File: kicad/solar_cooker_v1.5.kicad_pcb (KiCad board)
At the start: 2 copper layers, 160.5 x 77.2 mm, 20 parts, among them J1 Pt100, J2 microSD, J3 clock_module, J4 Pt100, J5 BME680, J6 GPS, J7 Pt100, J8 display, U1 anemometer, U2 AM2315C, U3 pyranometer

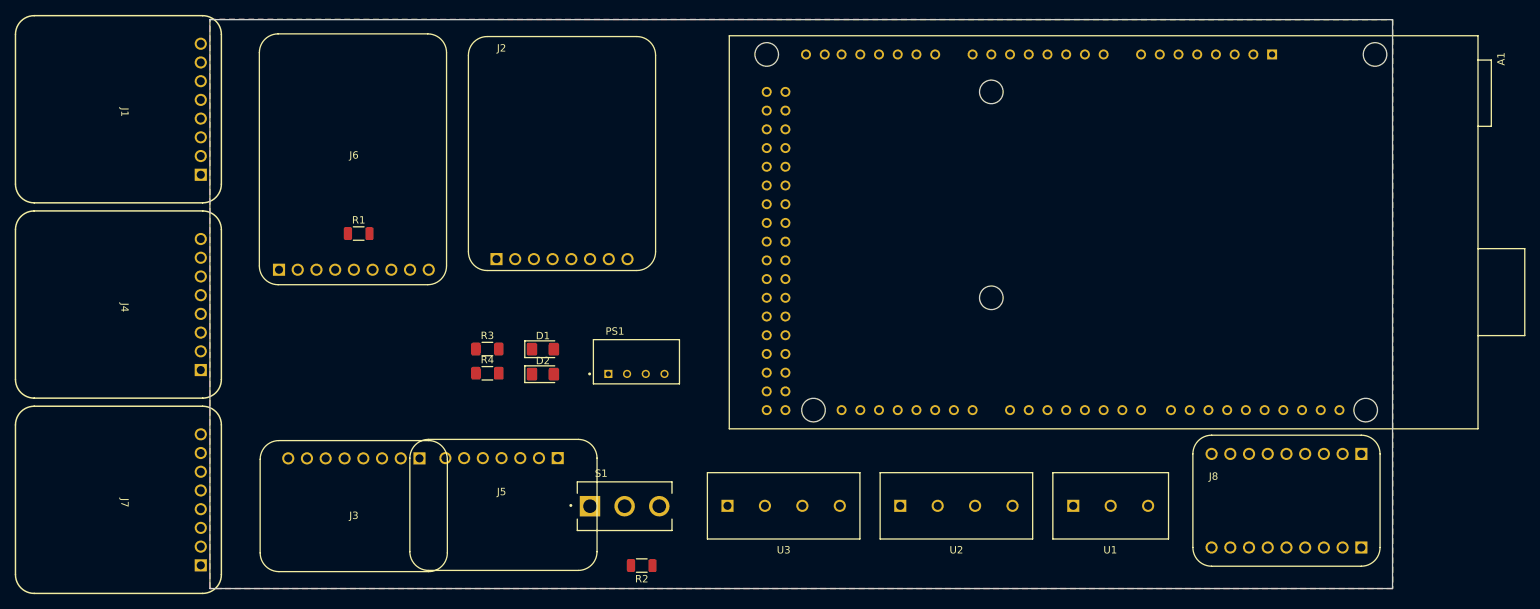
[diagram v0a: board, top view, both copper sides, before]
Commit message: all footprints ready
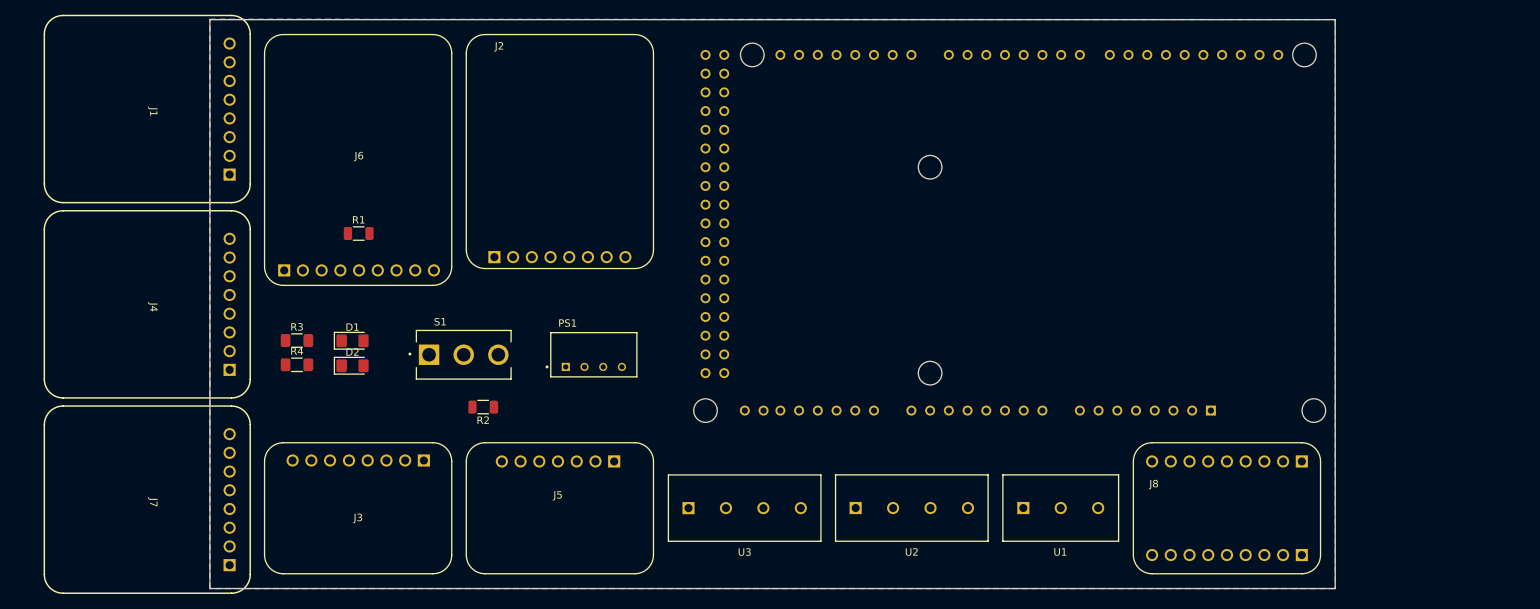
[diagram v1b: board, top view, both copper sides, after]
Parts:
- A1: moved to B.Cu
- moved R2 30.4 mm to (107.2, 132.6)
- moved S1 30.0 mm to (104.5, 125.5)
- moved R3 25.9 mm to (81.9, 123.5)
- moved R4 25.9 mm to (81.9, 126.8)
- moved D1 25.9 mm to (89.5, 123.6)
- moved D2 25.9 mm to (89.5, 127.0)
- moved A1 8.31 mm to (183.1, 108.9), turned to 90 degrees
- moved J8 8.14 mm to (208.1, 146.3)
- moved J5 7.67 mm to (117.3, 146.3)
- moved U1 6.78 mm to (185.6, 146.3)
- moved U2 6.06 mm to (165.3, 146.3)
- moved PS1 5.86 mm to (122.2, 125.5)
- moved U3 5.30 mm to (142.7, 146.3)
- moved J1 3.92 mm to (61.1, 92.1)
- moved J4 3.92 mm to (61.1, 118.6)
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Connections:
- J8 pad 1: /D3 -> +5V
- J8 pad 2: /D5 -> unconnected-(J8-Lite-Pad2)
- J8 pad 3: /D7 -> GND
- J8 pad 4: /MISO -> /SCK
- J8 pad 6: /SCK -> /MISO
- J8 pad 7: GND -> /D7
- J8 pad 8: unconnected-(J8-Lite-Pad8) -> /D5
- J8 pad 9: +5V -> /D3
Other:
- board size 160.5 x 77.2 mm -> 152.7 x 77.2 mm

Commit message: PCB routing and footprints done
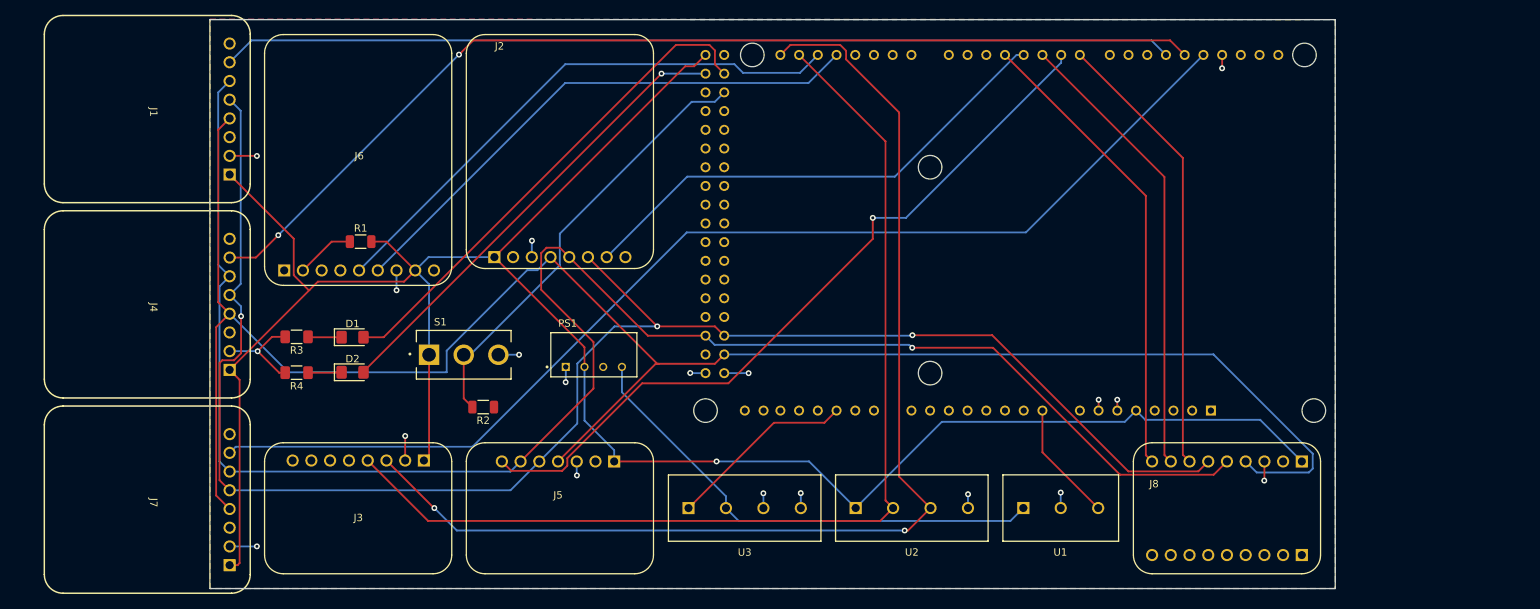
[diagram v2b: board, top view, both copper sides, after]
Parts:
- moved R1 1.13 mm to (90.5, 110.1)
- moved R4 1.07 mm to (81.9, 127.9), turned to 180 degrees
- moved D2 0.89 mm to (89.5, 127.9)
- moved R3 0.51 mm to (81.9, 123.0), turned to 180 degrees
- moved D1 0.48 mm to (89.5, 123.1)
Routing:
- net +5V: track 0.00 -> 303.9 mm, vias 0 -> 1
- net /SCK: track 0.00 -> 257.4 mm
- net /MOSI: track 0.00 -> 237.7 mm, vias 0 -> 1
- net /MISO: track 0.00 -> 226.4 mm, vias 0 -> 3
- net /SCL: track 0.00 -> 155.6 mm, vias 0 -> 2
- net /D13: track 0.00 -> 154.5 mm
- net /D12: track 0.00 -> 142.6 mm, vias 0 -> 2
- net /SDA: track 0.00 -> 142.2 mm
- net /D11: track 0.00 -> 129.1 mm
- net /D6: track 0.00 -> 102.7 mm, vias 0 -> 1
- net /RX1: track 0.00 -> 75.3 mm
- net /TX1: track 0.00 -> 74.4 mm
- net /D22: track 0.00 -> 68.1 mm
- net /D4: track 0.00 -> 68.0 mm
- net +9V: track 0.00 -> 66.8 mm
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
